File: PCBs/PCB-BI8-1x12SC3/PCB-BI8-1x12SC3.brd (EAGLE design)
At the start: 218.4 x 33 mm, 67 parts, among them IC2 PCA9685, IC3 PCA9685, IC4 MCP23017SS

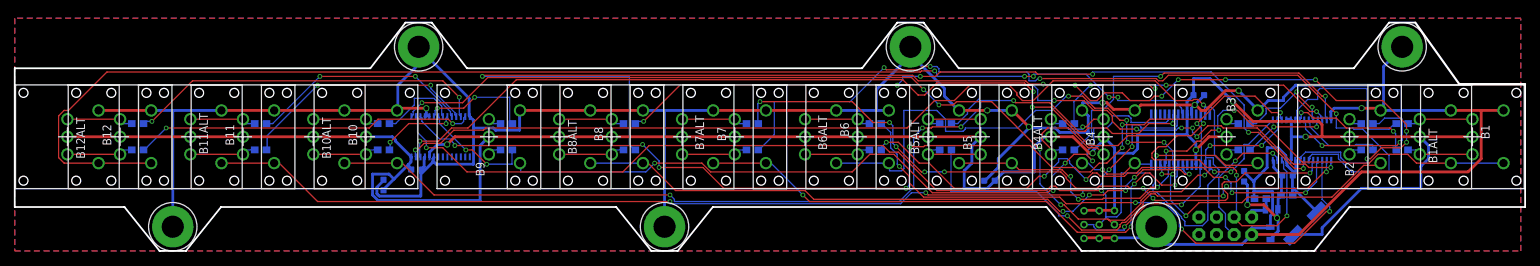
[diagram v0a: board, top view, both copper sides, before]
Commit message: Updates
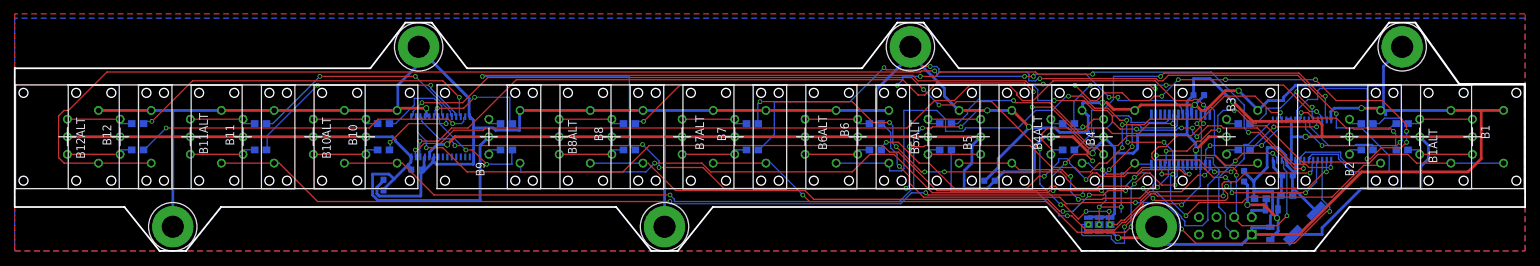
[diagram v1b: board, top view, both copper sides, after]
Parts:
- SERIAL: value M04X2 -> M04X2M2X4SMALLER; device SparkFun:2X4 -> SKAARHOJ:M2X4SMALLER
- U$19: value 3BITADDR -> 3BITADDRSMALL; device SKAARHOJ:3BITADDR -> SKAARHOJ:3BITADDR_SMALL
- turned SERIAL to 90 degrees
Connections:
- net 5V: now also U$19.H0; no longer U$19.H3
- net A0: now also U$19.AS0
- net A1: now also U$19.AS1
- net A2: now also U$19.AS2
- net GND: now also U$19.L0; no longer U$19.L3
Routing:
- net A2: track 176.6 -> 181.6 mm
- net A0: track 148.7 -> 150.2 mm, vias 8 -> 10
- net GND: track 462.9 -> 463.8 mm, vias 7 -> 8
- net A1: track 167.3 -> 168.0 mm, vias 4 -> 6
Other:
- board text added: "PCB-BI8-1x12SC3, v03-16"
- board text removed: "BI8-1x12SC3"
- board text removed: "Github: SKAARHOJ-Open-Engineering"
- board text removed: "SKAARHOJ 2015"
- board text removed: "v04-15"
